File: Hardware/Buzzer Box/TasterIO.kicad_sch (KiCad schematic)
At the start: 4 parts, among them J3 Conn_01x03_Socket, Q1 AO3400A, U3 LTV-817S

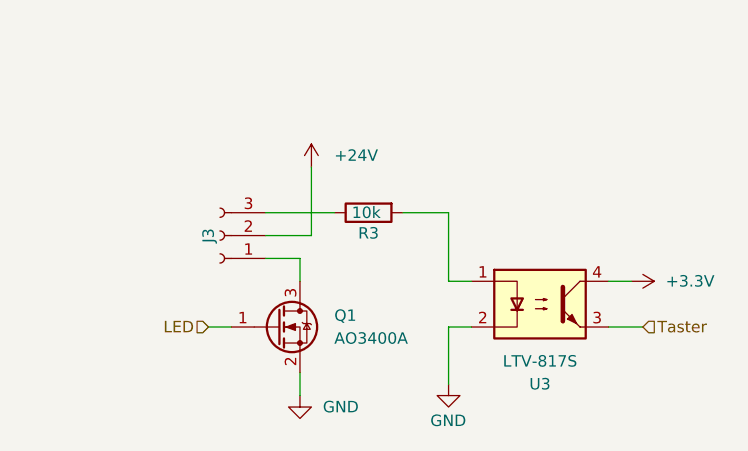
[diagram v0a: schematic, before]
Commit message: Updated the PCB
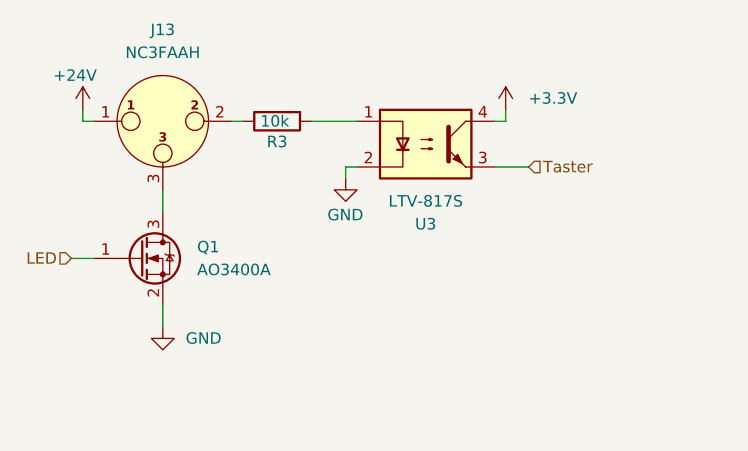
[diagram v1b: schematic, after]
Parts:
- removed J3: Conn_01x03_Socket, Connector_JST:JST_XH_B3B-XH-AM_1x03_P2.50mm_Vertical, symbol Connector:Conn_01x03_Socket
- added J13: NC3FAAH, Connector_Audio:Jack_XLR_Neutrik_NC3FAAH_Horizontal, symbol Connector_Audio:NC3FAAH
- R3: footprint Resistor_SMD:R_0805_2012Metric -> Resistor_SMD:R_0603_1608Metric
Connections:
- net +24V: now also J13.1
- net at Q1.3 (D): now also J13.3
- net at R3.1: now also J13.2
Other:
- moved on the sheet: Q1, R3, U3
